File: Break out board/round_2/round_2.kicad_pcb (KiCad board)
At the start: 2 copper layers, 2 parts, among them U1 LSM90S1

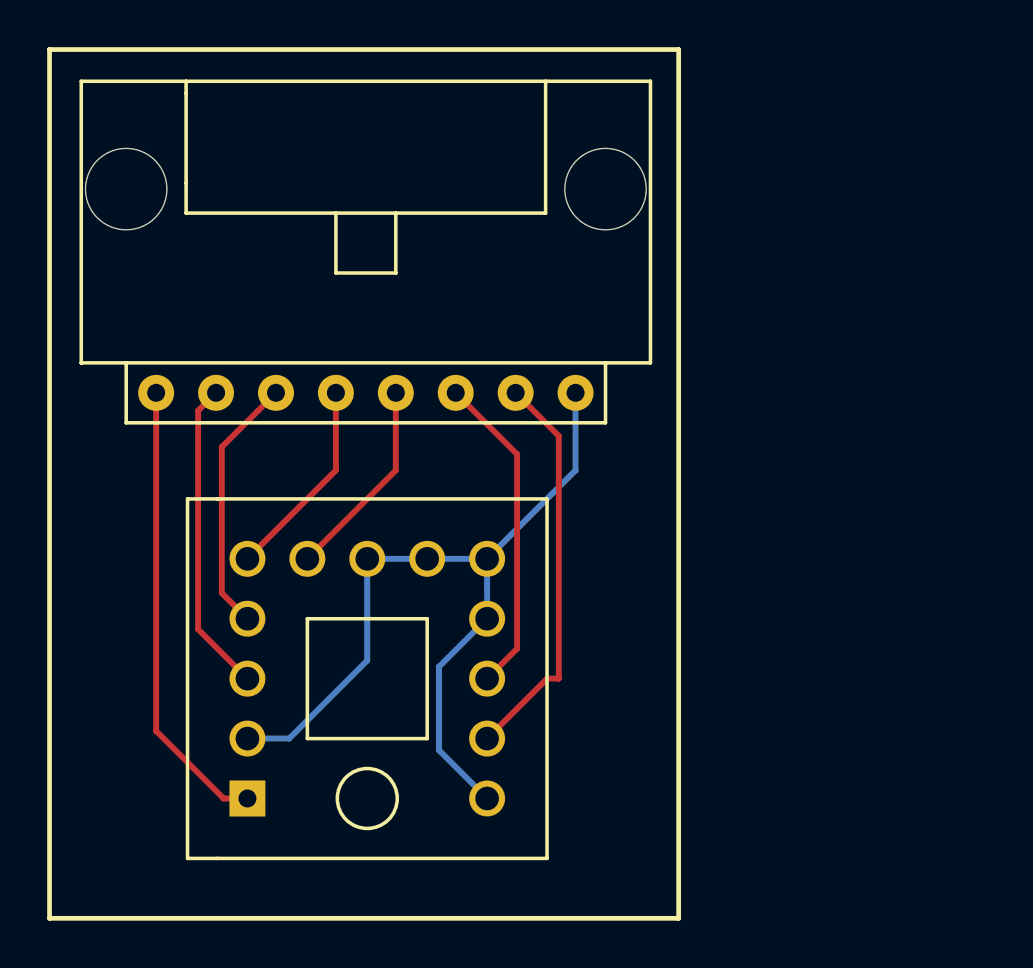
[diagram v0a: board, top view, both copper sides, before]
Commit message: Did everything
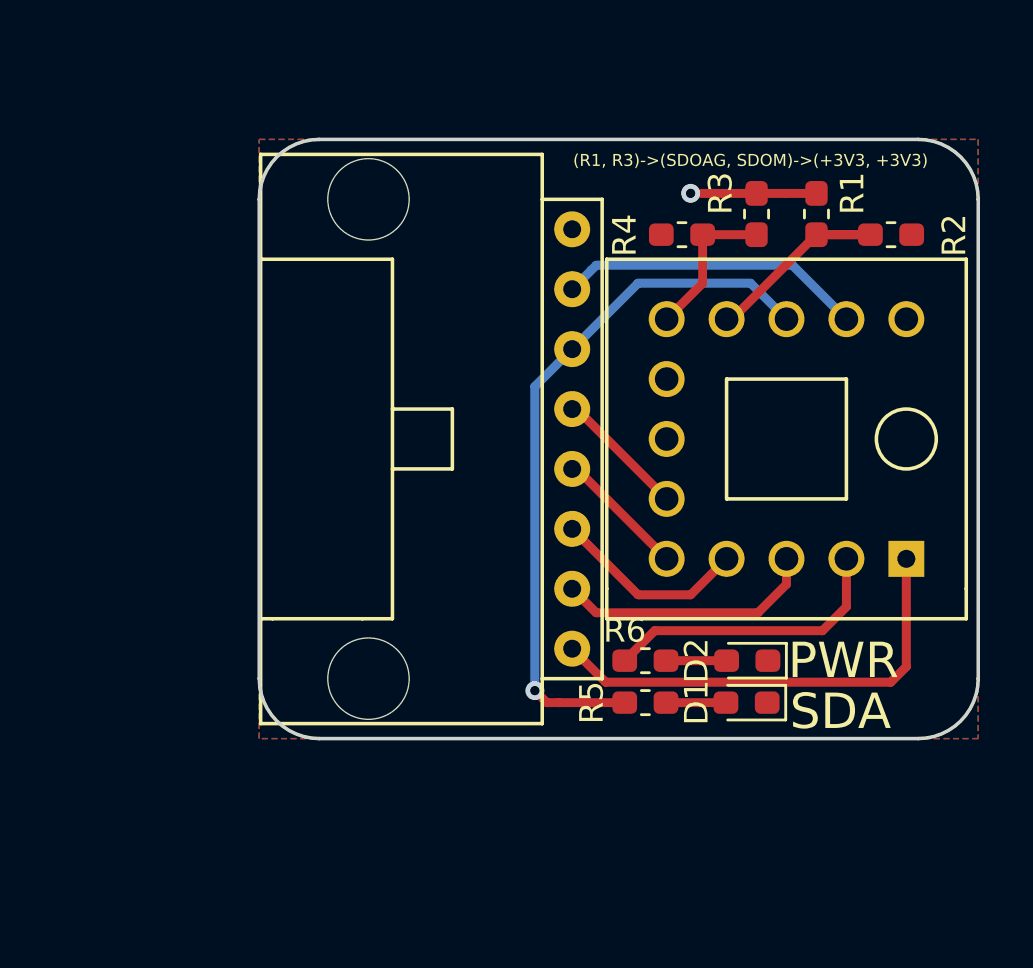
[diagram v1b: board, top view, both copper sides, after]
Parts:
- added D1: D, Diode_SMD:D_0603_1608Metric_Pad1.05x0.95mm_HandSolder, F.Cu at (155.3, 110.2)
- added D2: D, Diode_SMD:D_0603_1608Metric_Pad1.05x0.95mm_HandSolder, F.Cu at (155.3, 108.5)
- added G***: LOGO, MRDT_Silkscreens:MRDT_Logo_10mm, B.Cu at (159.6, 97.9)
- added R1: 0, Resistor_SMD:R_0603_1608Metric_Pad1.05x0.95mm_HandSolder, F.Cu at (158.2, 89.5)
- added R2: 1K, Resistor_SMD:R_0603_1608Metric_Pad1.05x0.95mm_HandSolder, F.Cu at (161.4, 90.4)
- added R3: 0, Resistor_SMD:R_0603_1608Metric_Pad1.05x0.95mm_HandSolder, F.Cu at (155.7, 89.5)
- added R4: 1K, Resistor_SMD:R_0603_1608Metric_Pad1.05x0.95mm_HandSolder, F.Cu at (152.5, 90.4)
- added R5: 500, Resistor_SMD:R_0603_1608Metric_Pad1.05x0.95mm_HandSolder, F.Cu at (151.0, 110.2)
- added R6: 500, Resistor_SMD:R_0603_1608Metric_Pad1.05x0.95mm_HandSolder, F.Cu at (151.0, 108.5)
- moved U1 10.5 mm to (149.4, 91.4), turned to 270 degrees
- moved Conn1 8.96 mm to (147.9, 99.1), turned to 90 degrees
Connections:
- net Net-(Conn1-Pad1) renamed GND
- net Net-(Conn1-Pad2) renamed INT2AG
- net Net-(Conn1-Pad3) renamed INT1AG
- net Net-(Conn1-Pad4) renamed INTM
- net Net-(Conn1-Pad5) renamed DRDYM
- net Net-(Conn1-Pad6) renamed SDA
- net Net-(Conn1-Pad7) renamed SCL
- Conn1 pad 8: Net-(Conn1-Pad8) -> +3V3
- U1 pad 1: Net-(Conn1-Pad8) -> +3V3
- U1 pad 12: Net-(Conn1-Pad8) -> +3V3
- U1 pad 4: Net-(Conn1-Pad8) -> SDOAG
- U1 pad 5: Net-(Conn1-Pad8) -> SDOM
- U1 pad 6: Net-(Conn1-Pad8) -> +3V3
- U1 pad 7: Net-(Conn1-Pad8) -> +3V3
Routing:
- net Net-(Conn1-Pad8): track 36.3 -> 0.00 mm
- net +3V3: track 0.00 -> 17.7 mm, vias 0 -> 1
- net SDA: track 13.7 -> 30.0 mm, vias 0 -> 1
- net SDOAG: track 0.00 -> 9.61 mm
- net SDOM: track 0.00 -> 6.50 mm
- net SCL: track 17.0 -> 13.0 mm
- net DRDYM: track 8.59 -> 5.39 mm
- net INTM: track 8.59 -> 5.39 mm
- net INT1AG: track 11.0 -> 8.33 mm
- net Net-(D2-Pad2): track 0.00 -> 2.54 mm
- net Net-(D1-Pad2): track 0.00 -> 2.54 mm
- net INT2AG: track 13.3 -> 11.1 mm
- added copper zone on B.Cu, net +3V3
- added copper zone on F.Cu, net GND
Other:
- board outline added: 30.5 x 25.4 mm
- board text added: "(R1, R3)->(SDOAG, SDOM)->(+3V3, +3V3)"
- board text added: "IMU Breakout, Rev 1 Mars Rover, 2019 Missouri S&T"
- board text added: "PWR"
- board text added: "SDA"
